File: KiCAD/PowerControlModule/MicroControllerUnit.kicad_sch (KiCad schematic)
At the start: 3 parts, among them U1 XIAO-RP2040-DIP

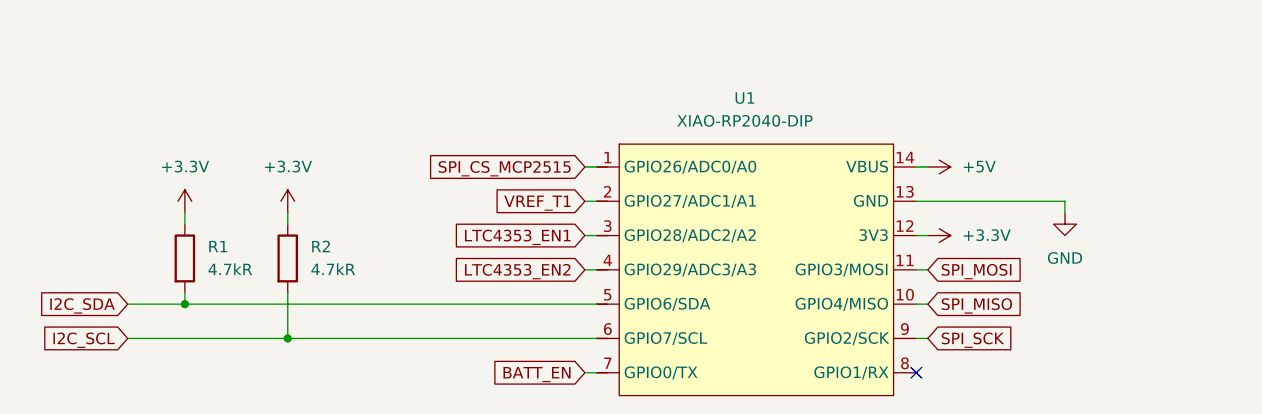
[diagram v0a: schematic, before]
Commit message: Build-5を作成
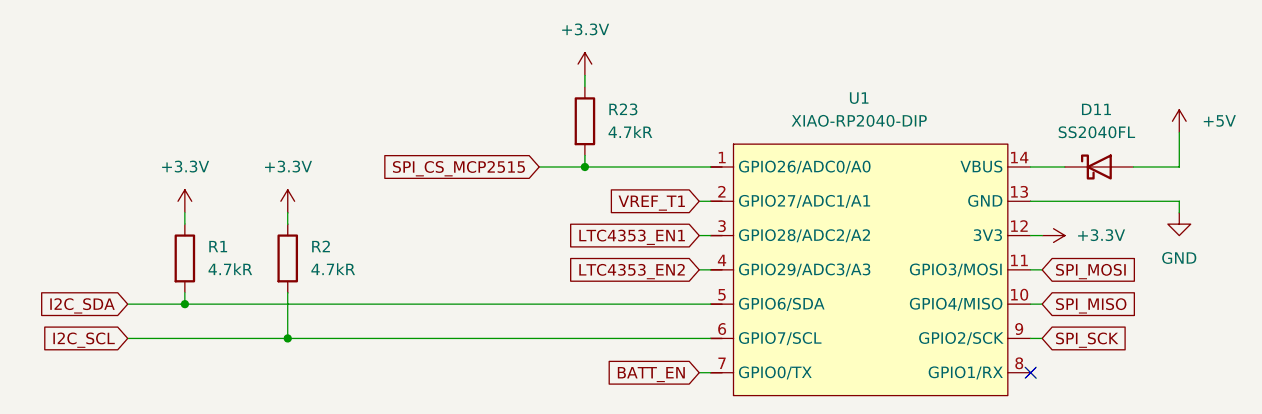
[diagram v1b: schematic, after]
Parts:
- added D11: SS2040FL, Diode_SMD:D_SOD-123F, symbol Device:D_Schottky
- added R23: 4.7kR, Resistor_SMD:R_0603_1608Metric_Pad0.98x0.95mm_HandSolder, symbol Device:R
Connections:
- net +3.3V: now also R23.1
- net +5V: now also D11.2 (A); no longer U1.14 (VBUS)
- net SPI_CS_MCP2515: now also R23.2
- new net: D11.1 (K), U1.14 (VBUS)
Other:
- moved on the sheet: U1
